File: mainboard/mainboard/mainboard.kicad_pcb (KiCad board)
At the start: 2 copper layers, 1 part

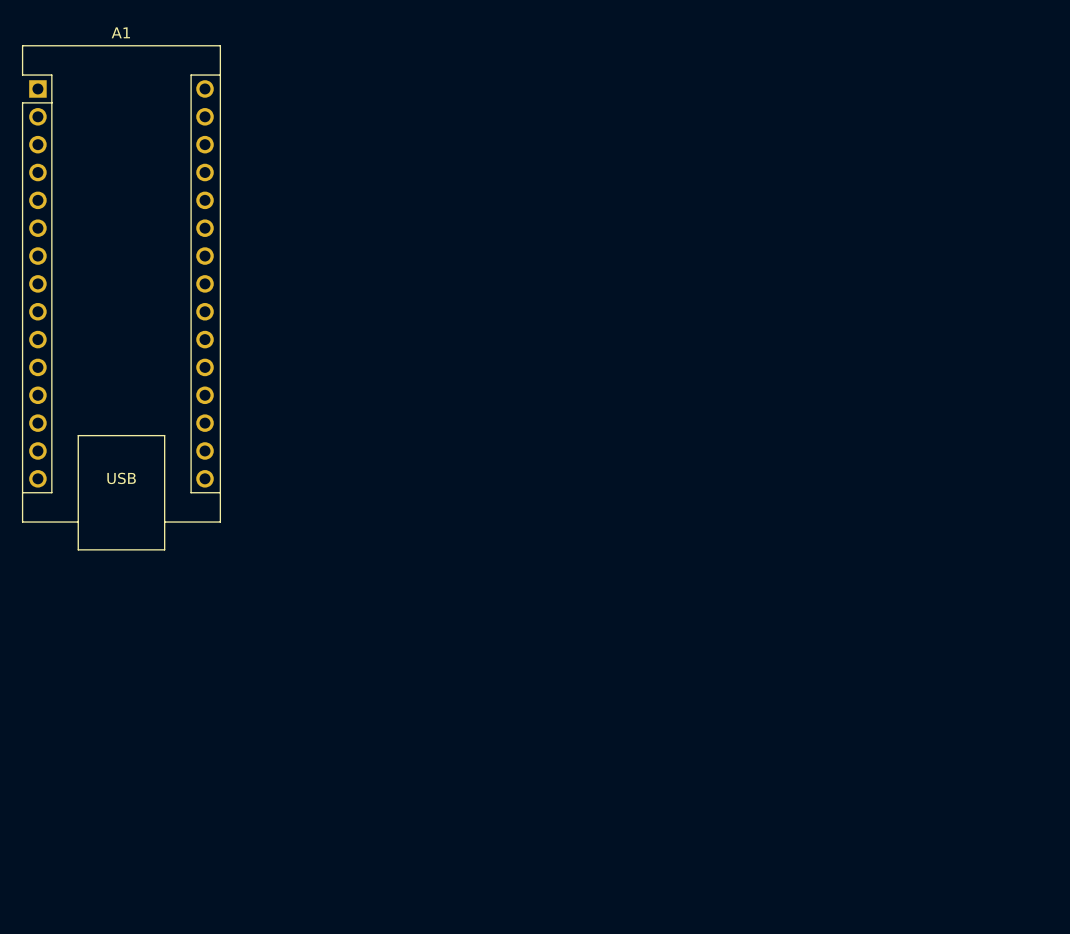
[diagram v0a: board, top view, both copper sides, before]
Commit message: added gerber files
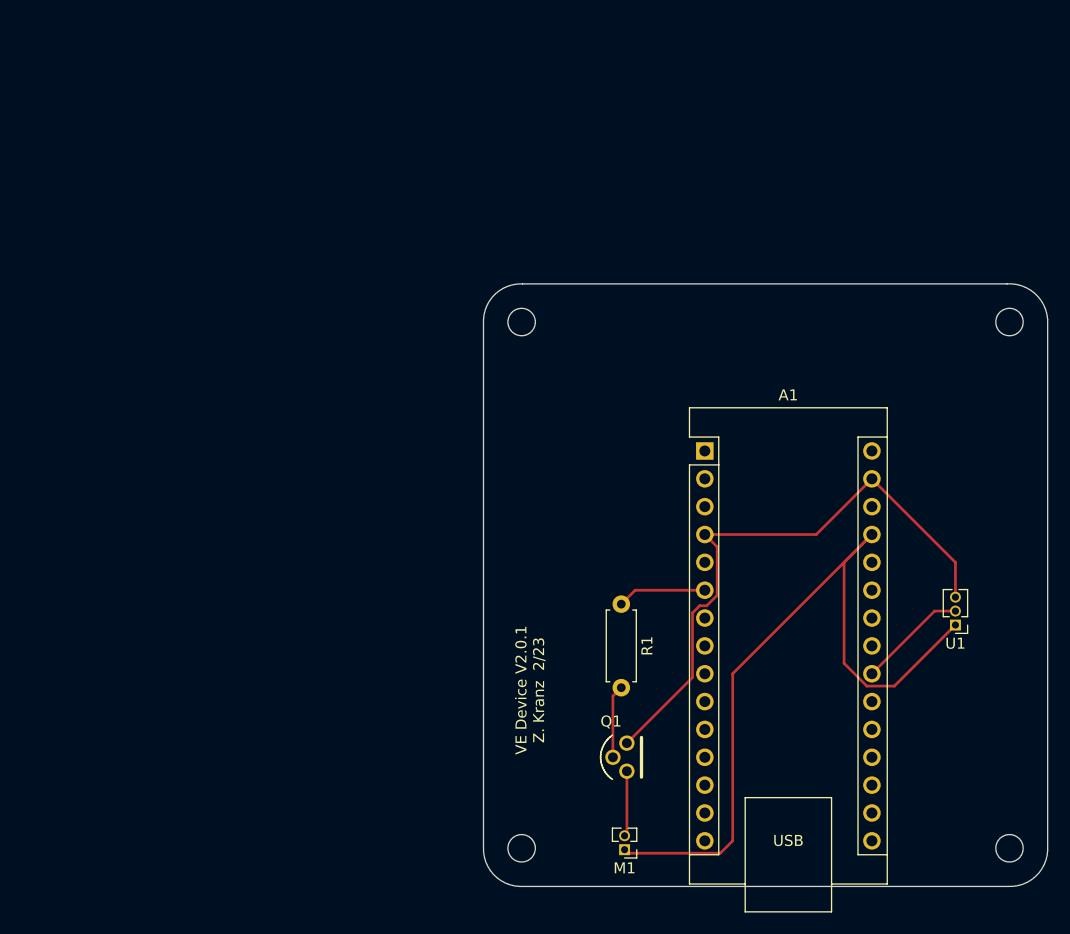
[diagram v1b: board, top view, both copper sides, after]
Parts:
- added M1: Motor_DC, Connector_PinHeader_1.27mm:PinHeader_1x02_P1.27mm_Vertical, F.Cu at (109.4, 148.1)
- added Q1: P2N2222A, vision-empower:ON_Semi-CASE_2911-0-0-0, F.Cu at (109.1, 139.7)
- added R1: 1k, Resistor_THT:R_Axial_DIN0207_L6.3mm_D2.5mm_P7.62mm_Horizontal, F.Cu at (109.1, 125.7)
- added REF**: MountingHole_2.5mm, MountingHole:MountingHole_2.5mm, F.Cu at (144.5, 148.0)
- added REF**: MountingHole_2.5mm, MountingHole:MountingHole_2.5mm, F.Cu at (100.0, 148.0)
- added REF**: MountingHole_2.5mm, MountingHole:MountingHole_2.5mm, F.Cu at (144.5, 100.0)
- added REF**: MountingHole_2.5mm, MountingHole:MountingHole_2.5mm, F.Cu at (100.0, 100.0)
- added U1: LS_CONN, Connector_PinHeader_1.27mm:PinHeader_1x03_P1.27mm_Vertical, F.Cu at (139.6, 127.6)
- moved A1 69.2 mm to (116.7, 111.8)
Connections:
- net Net-(A1-Pad29) renamed GND
- A1 pad 22: unconnected-(A1-Pad22) -> Net-(A1-Pad22)
- A1 pad 27: unconnected-(A1-Pad27) -> +5V
- A1 pad 6: unconnected-(A1-Pad6) -> T1
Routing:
- net +5V: track 0.00 -> 69.8 mm
- net GND: track 0.00 -> 54.6 mm
- net Net-(A1-Pad22): track 0.00 -> 9.99 mm
- net T1: track 0.00 -> 8.15 mm
- net Net-(R1-Pad2): track 0.00 -> 6.67 mm
- net Net-(Q1-Pad1): track 0.00 -> 5.97 mm
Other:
- board outline added: 51.5 x 55 mm
- board text added: "VE Device V2.0.1 Z. Kranz 2/23"
